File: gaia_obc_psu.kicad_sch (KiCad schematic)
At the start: 68 parts, among them Q2 FS8205A, SW8 SW_Slide_DPDT, U10 TPS22917DBV, U11 AP2112K-3.3, U12 DW01A, U13 AP2112K-3.0, U14 LGS4056HDB, U19 INA238/INA237, U4 INA3221, U5 INA3221, U6 TPS22917DBV, U7 TPS22917DBV, U8 TPS22917DBV, U9 TPS22917DBV

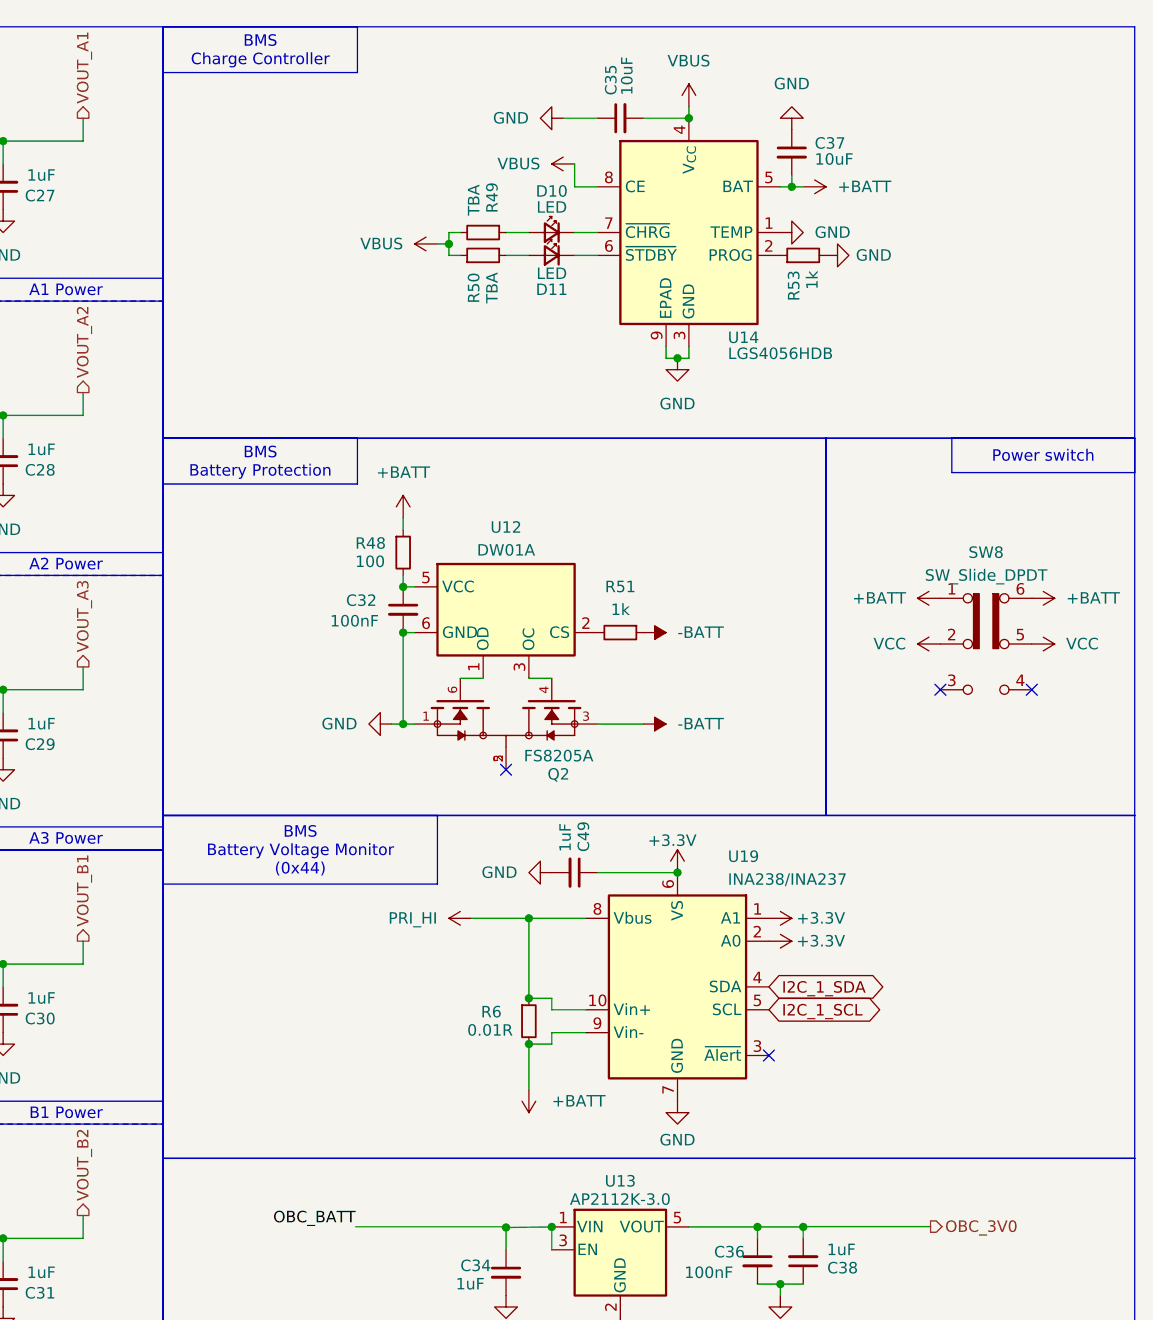
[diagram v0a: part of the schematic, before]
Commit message: v1.3
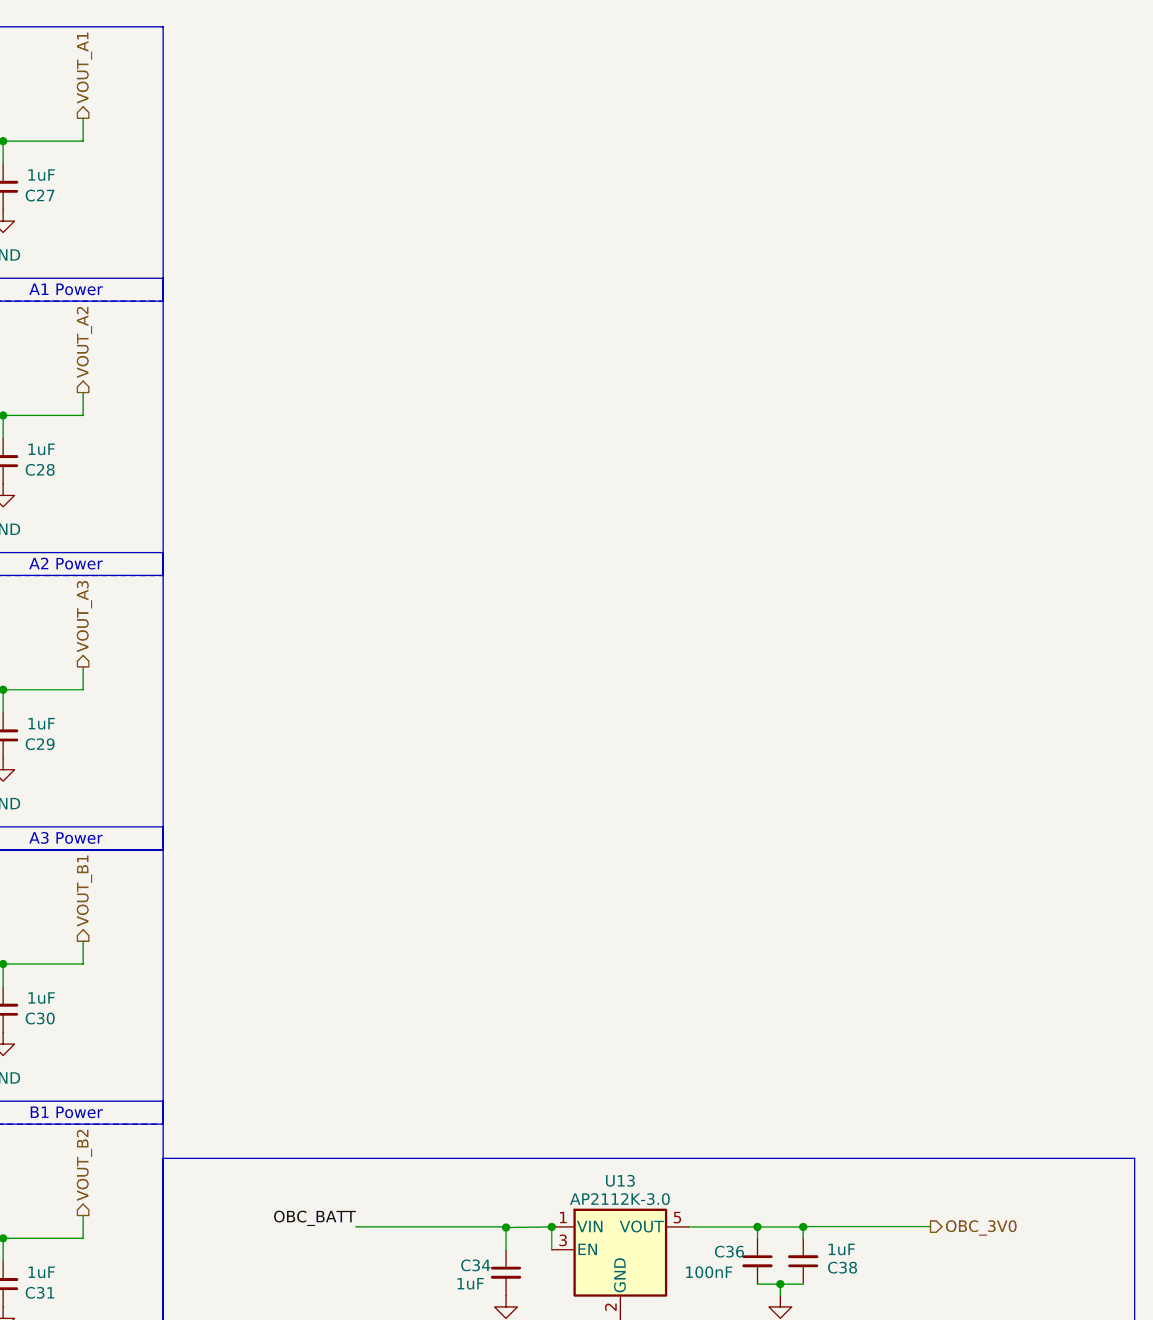
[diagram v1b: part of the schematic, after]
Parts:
- removed C32: 100nF, Capacitor_SMD:C_0402_1005Metric, symbol Device:C_Small
- removed C35, C37: 10uF, Capacitor_SMD:C_0603_1608Metric, symbol Device:C_Small
- removed C49: 1uF, Capacitor_SMD:C_0603_1608Metric, symbol Device:C_Small
- removed D10, D11: LED, LED_SMD:LED_0805_2012Metric, symbol Device:LED_Small
- removed Q2: FS8205A, gaia_obc-footprints:SOT-23-6, symbol OnionSAT_Gaia:FS8205A
- removed R48: 100, Resistor_SMD:R_0603_1608Metric, symbol Device:R_Small
- removed R49, R50: TBA, Resistor_SMD:R_0402_1005Metric, symbol Device:R_Small
- removed R51: 1k, Resistor_SMD:R_0603_1608Metric, symbol Device:R_Small
- removed R53: 1k, Resistor_SMD:R_0402_1005Metric, symbol Device:R_Small
- removed R6: 0.01R, Resistor_SMD:R_2512_6332Metric, symbol Device:R_Small
- removed SW8: SW_Slide_DPDT, gaia_obc-footprints:MS-22D28-G020, symbol Switch:SW_Slide_DPDT
- removed U12: DW01A, gaia_obc-footprints:SOT-23-6, symbol Battery_Management:DW01A
- removed U14: LGS4056HDB, gaia_obc-footprints:DFN-8-1EP_3x3mm_P0.65mm_EP1.55x2.4mm, symbol gaia_obc-symbols:LGS4056HDB
- removed U19: INA238/INA237, Package_SO:VSSOP-10_3x3mm_P0.5mm, symbol Sensor_Energy:INA238
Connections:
- no-connect marks 4 -> 0

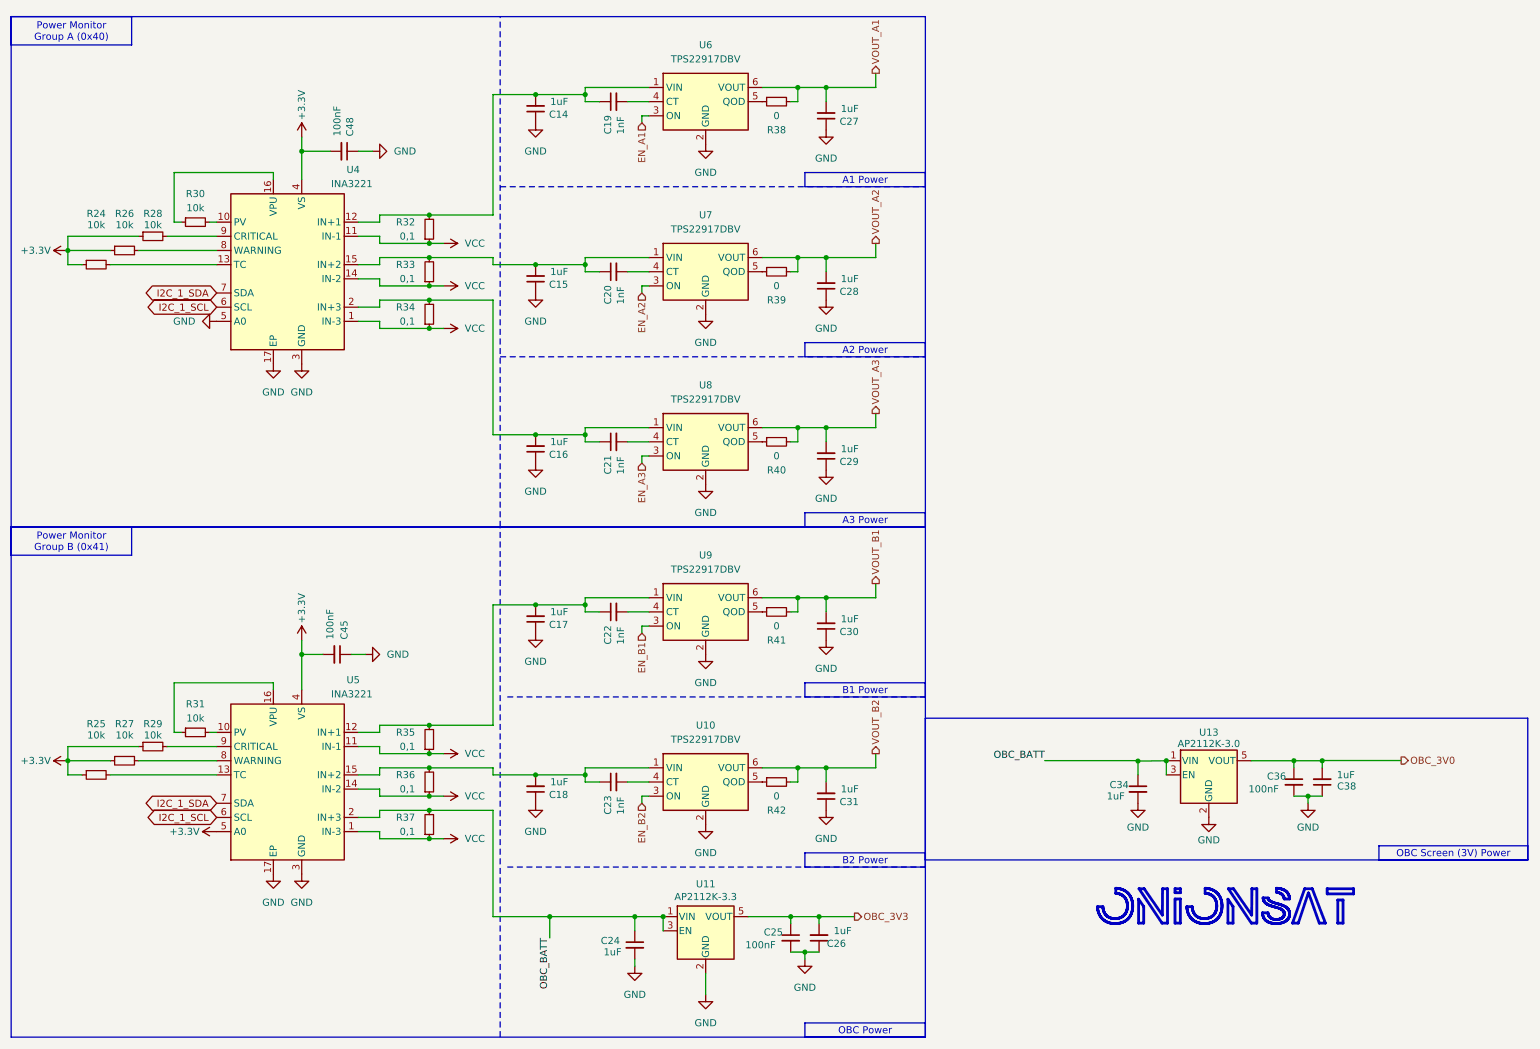
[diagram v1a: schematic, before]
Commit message: neptune 1.3 production
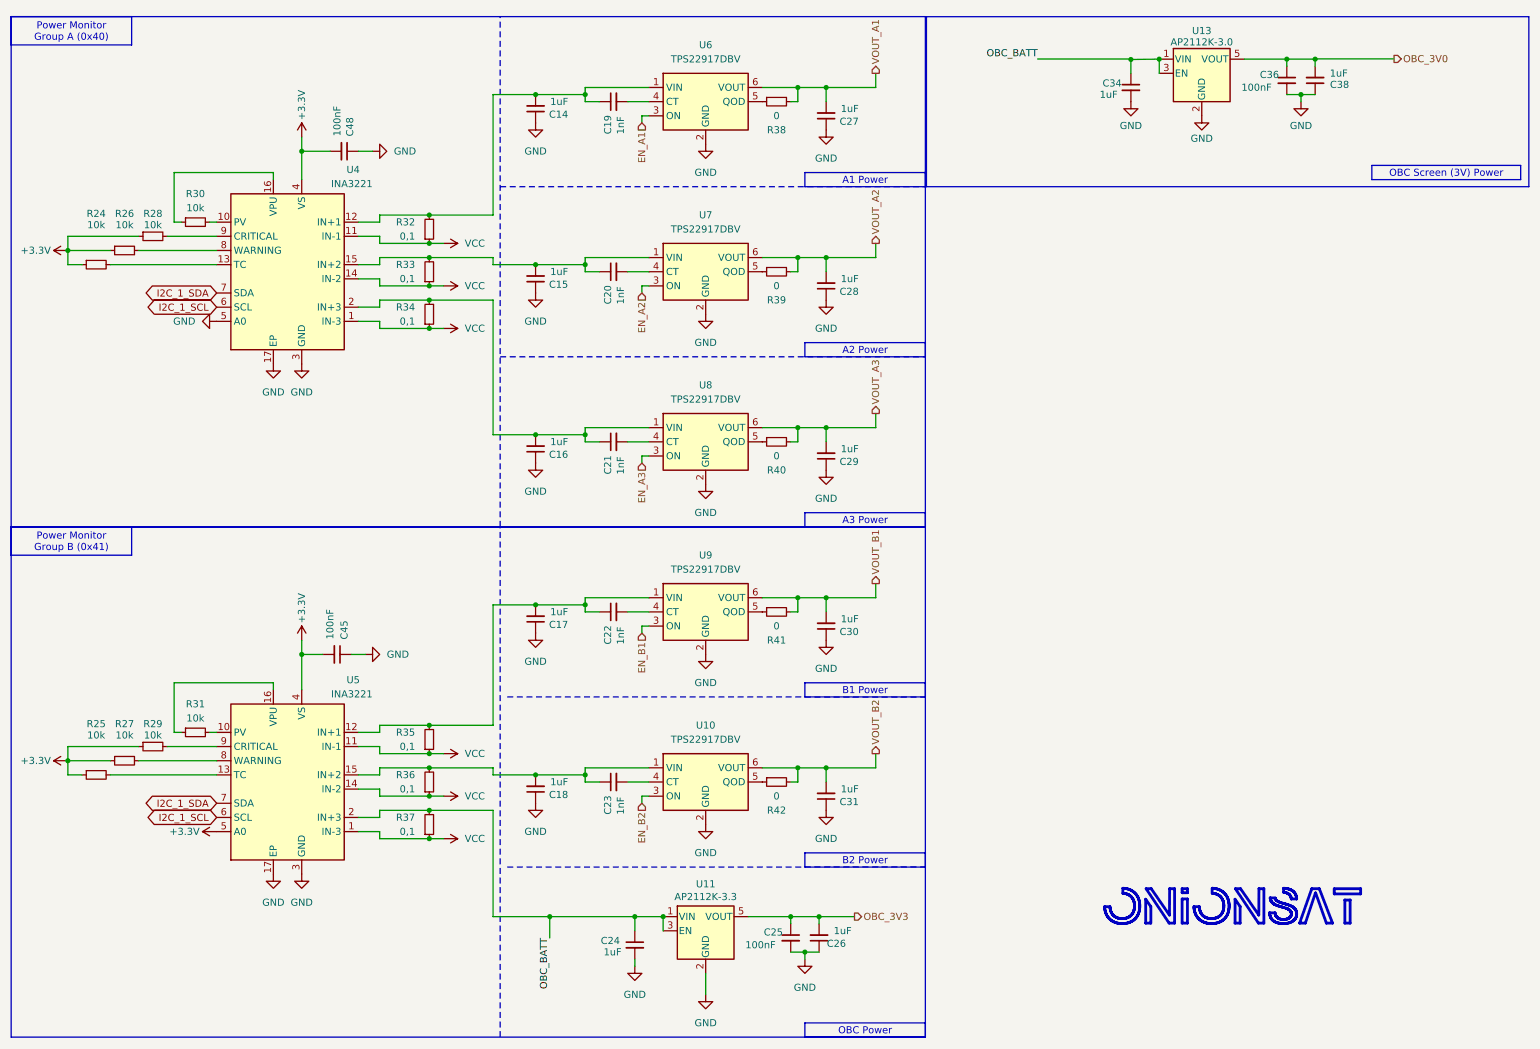
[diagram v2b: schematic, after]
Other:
- title: GAIA On-Board Computer -> Neptune On-Board Computer
- moved on the sheet: C34, C36, C38, U13
